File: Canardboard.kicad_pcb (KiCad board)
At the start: 4 copper layers, 50.7 x 58.7 mm, 170 parts, among them IC1 SIC437DED-T1-GE3, J1 RBUS, J2 USB_C_Receptacle_USB2.0, J3 Micro_SD_Card_Det, J4 Conn_01x02_Male, J5 Conn_01x03_Male, J6 Conn_01x03_Male, J7 Conn_01x03_Male, Q1 PXP012-30QLJ, Q2 PXP012-30QLJ, Q4 PXP012-30QLJ, Q6 PXP012-30QLJ, U1 ESP32-S3, U10 MP28167GQ-A-Z, U2 SN65HVD230, U3 LTC4412xS6, U4 LTC4412xS6, U5 74AHC1G00, U6 74AHC1G08, U7 ICM-20608-G, U8 MMC5983MA, U9 SC4215, Y1 40MHz±10ppm

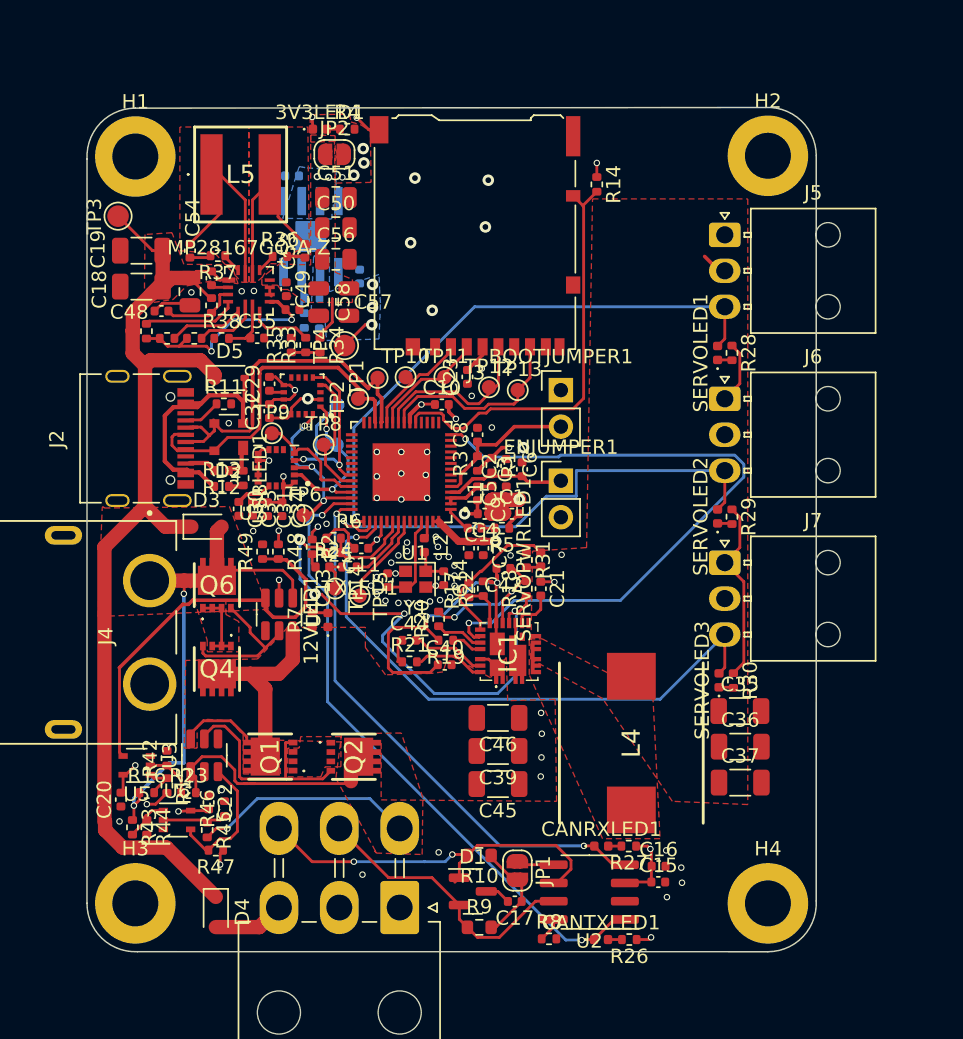
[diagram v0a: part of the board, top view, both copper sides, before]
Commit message: did some stuffus
added a new power plane in servo power on the back side
made SW larger
and a lot more changes
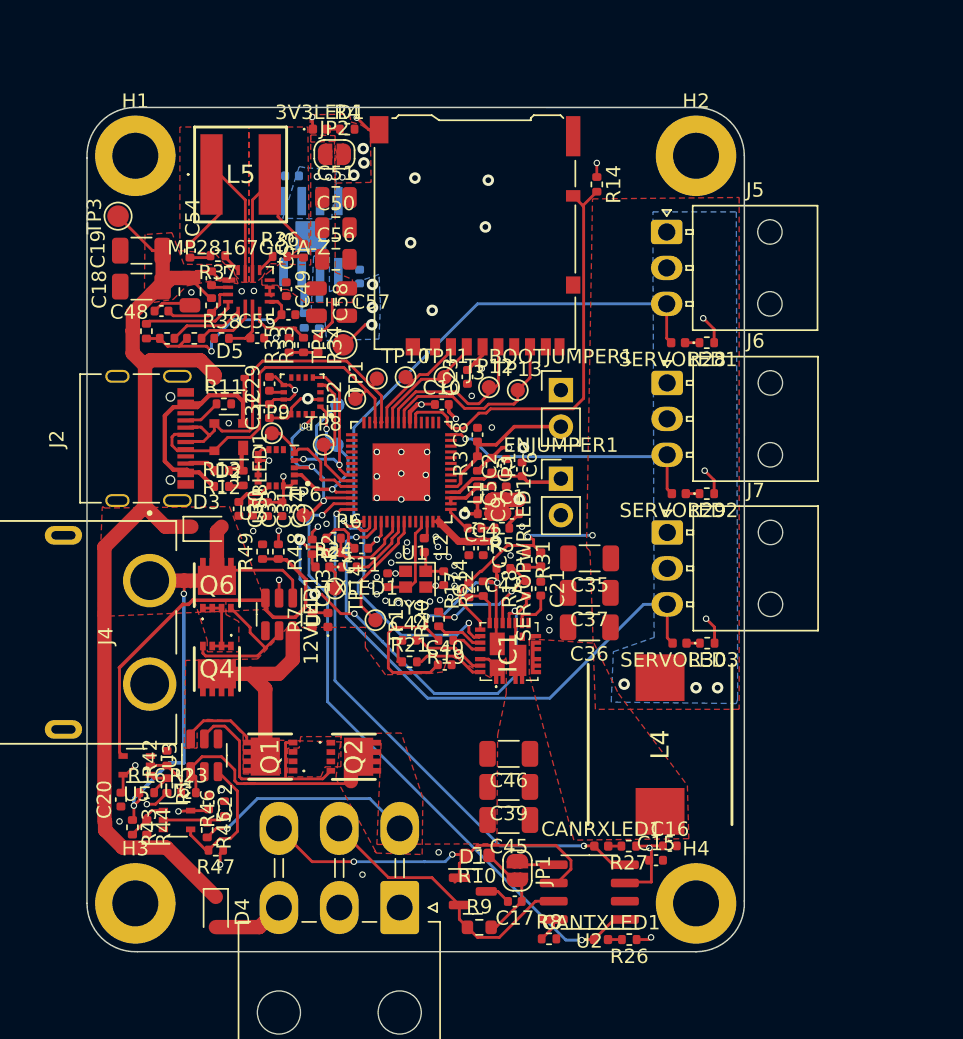
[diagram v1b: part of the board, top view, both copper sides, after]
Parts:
- moved C37 16.9 mm to (135.6, 105.4), turned to 180 degrees
- moved C35 14.9 mm to (135.6, 103.0), turned to 180 degrees
- moved C36 13.4 mm to (135.6, 107.8), turned to 180 degrees
- moved H2 5.00 mm to (143.0, 75.0)
- moved H4 5.00 mm to (143.0, 127.0)
- moved J7 4.52 mm to (141.0, 101.2)
- moved J6 4.16 mm to (141.0, 90.8)
- moved J5 4.04 mm to (141.0, 80.3)
- moved SERVOLED3 3.77 mm to (141.9, 108.9), turned to 180 degrees
- moved R30 3.17 mm to (143.8, 108.9), turned to 180 degrees
- moved SERVOLED2 3.13 mm to (141.8, 98.5), turned to 180 degrees
- moved SERVOLED1 2.84 mm to (141.8, 88.0), turned to 180 degrees
- moved C39 2.61 mm to (130.0, 118.9)
- moved C45 2.61 mm to (130.0, 121.2)
- moved C46 2.61 mm to (130.0, 116.6)
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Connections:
- U1 pad 14: /SERVOBUCK_EN -> /SERVO_SGNL2
- U1 pad 44: /SERVO_SGNL2 -> /SERVOBUCK_EN
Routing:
- net /SERVOBUCK_EN: track 47.4 -> 19.8 mm
- net /SERVO_SGNL2: track 35.0 -> 18.6 mm
- net GND: track 54.8 -> 42.3 mm, vias 71 -> 67
- net /SERVO_PWR: track 11.8 -> 16.4 mm, vias 0 -> 5
- net /SERVO_SGNL1: track 39.3 -> 35.2 mm
- net /servopower/PGOOD: track 34.9 -> 31.5 mm
- net /SERVO_SGNL3: track 41.6 -> 38.4 mm
- net /RXD: track 5.91 -> 8.52 mm
- net /servopower/uC_VCC: track 15.1 -> 13.9 mm
- net +3.3V: track 48.0 -> 49.0 mm
- net /Data-: track 25.6 -> 24.9 mm
- added copper zone on B.Cu, net /SERVO_PWR
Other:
- board size 50.7 x 58.7 mm -> 45.7 x 58.7 mm
